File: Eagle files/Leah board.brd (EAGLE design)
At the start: 43.2 x 43.2 mm, 10 parts

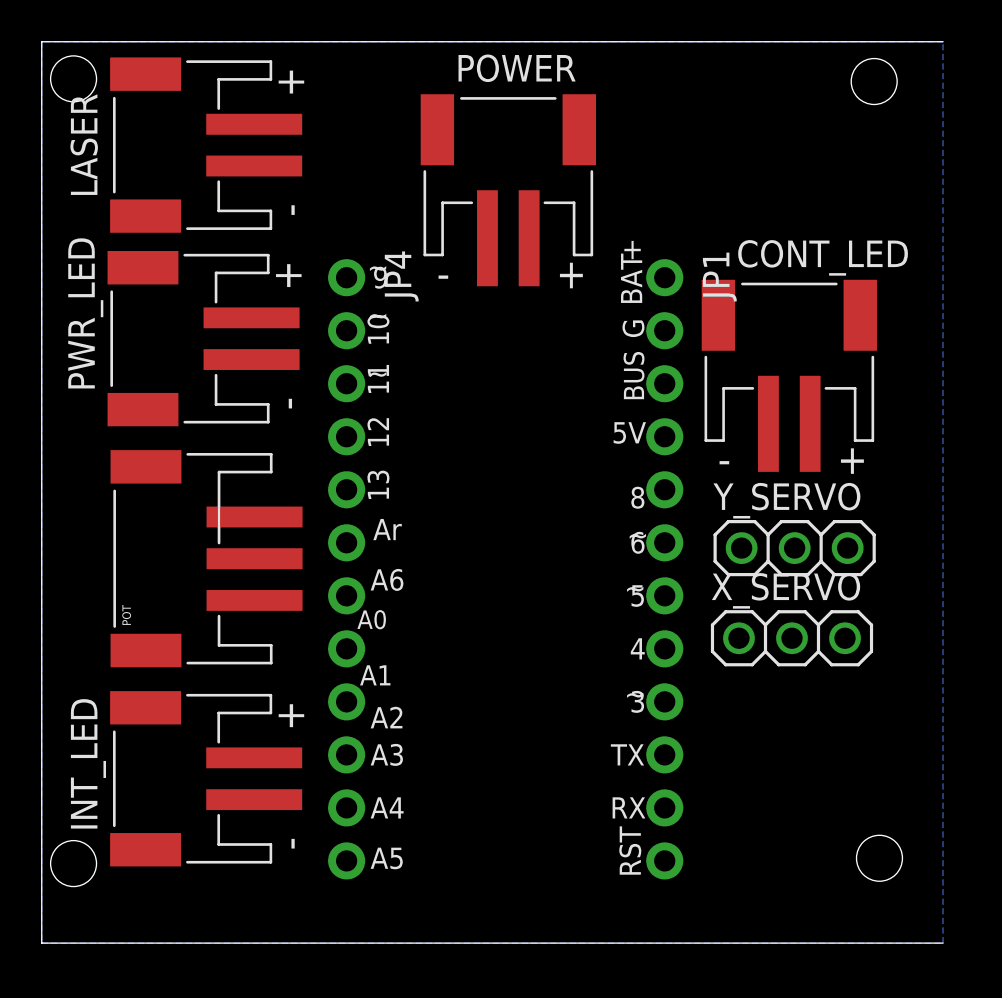
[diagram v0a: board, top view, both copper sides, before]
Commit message: Modification for present.
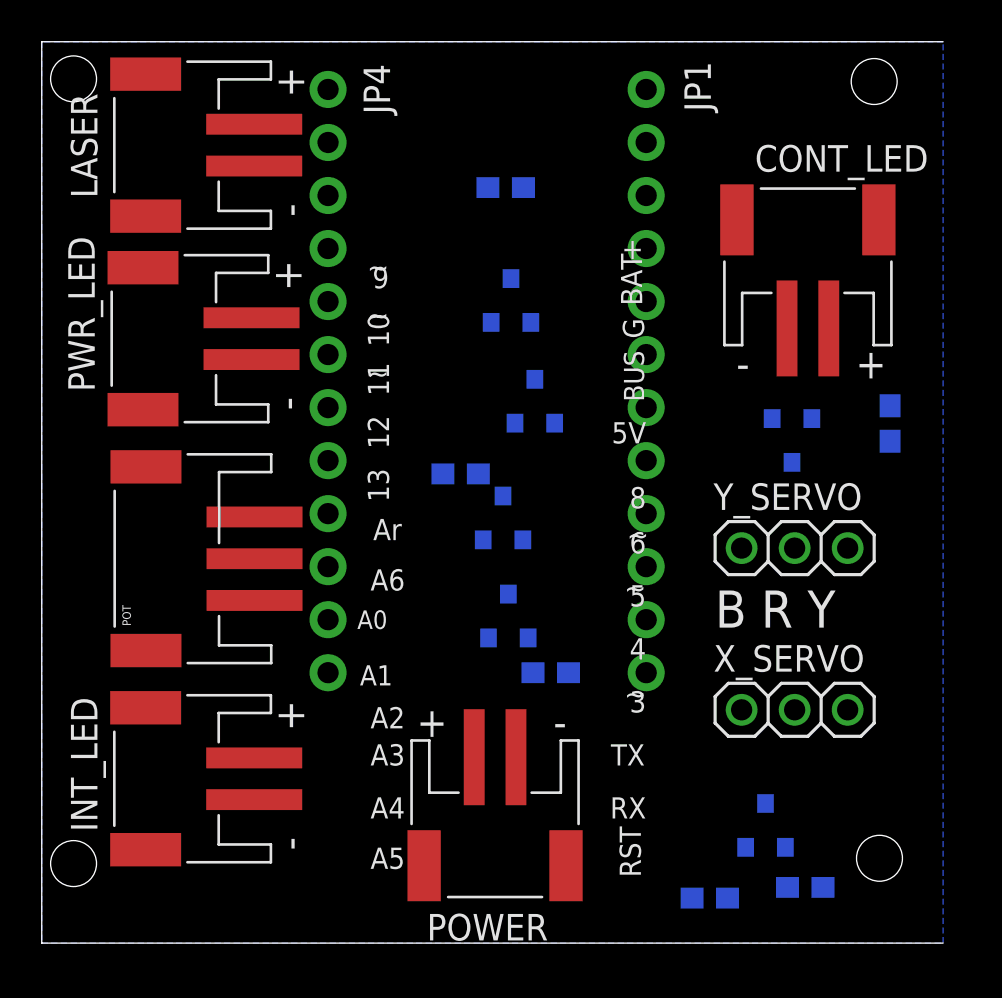
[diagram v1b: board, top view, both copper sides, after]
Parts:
- added CONT_MOS, INT_MOS, LASER_MOS, PWR_MOS, X_MOS, Y_MOS: 200mA/50V, SparkFun-DiscreteSemi:SOT23-3
- added R1, R2, R3, R4, R5, R6: 10K, SparkFun-Resistors:0603-RES
- moved POWER 32.3 mm to (21.7, 5.21), turned to 180 degrees
- moved JP1 9.06 mm to (29.0, 26.9)
- moved JP4 9.06 mm to (13.7, 26.9)
- moved CONT_LED 4.66 mm to (36.7, 33.1)
- moved X_SERVO 3.43 mm to (36.1, 11.2)
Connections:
- new net CONT_PWR: CONT_LED.1, CONT_MOS.2, R2.2
- new net INT_PWR: INT_LED.1, INT_MOS.2, R1.2
- new net LASER_PIN: LASER_MOS.1
- new net N$2: INT_MOS.1
- new net N$3: CONT_MOS.1
- new net N$4: PWR_MOS.1
- new net N$5: LASER_MOS.2, R4.2
- new net N$6: R6.2, Y_MOS.2, Y_SERVO.2
- new net N$7: R5.2, X_MOS.2, X_SERVO.2
- new net PLED_PWR: PWR_LED.1, PWR_MOS.2, R3.2
- new net XSERVO_PWR_PIN: X_MOS.1
- new net YSERVO_PWR_PIN: Y_MOS.1
- net A0: now also X_SERVO.3
- net A1: now also Y_SERVO.1
- net GND: now also CONT_LED.2, INT_LED.2, POT.3, PWR_LED.2, R1.1, R2.1, R3.1, R4.1, R5.1, R6.1, X_SERVO.1, Y_SERVO.3
- net VCC: now also CONT_MOS.3, INT_MOS.3, LASER_MOS.3, POT.1, PWR_MOS.3, X_MOS.3, Y_MOS.3
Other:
- board text added: "B R Y"
